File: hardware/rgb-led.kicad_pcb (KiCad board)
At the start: 2 copper layers, 20 x 25 mm, 22 parts, among them P1 CON-SENSOR, Q1 2N7002P, U1 M24C64, U2 DRILL, U3 DRILL, U4 DRILL, U5 DRILL

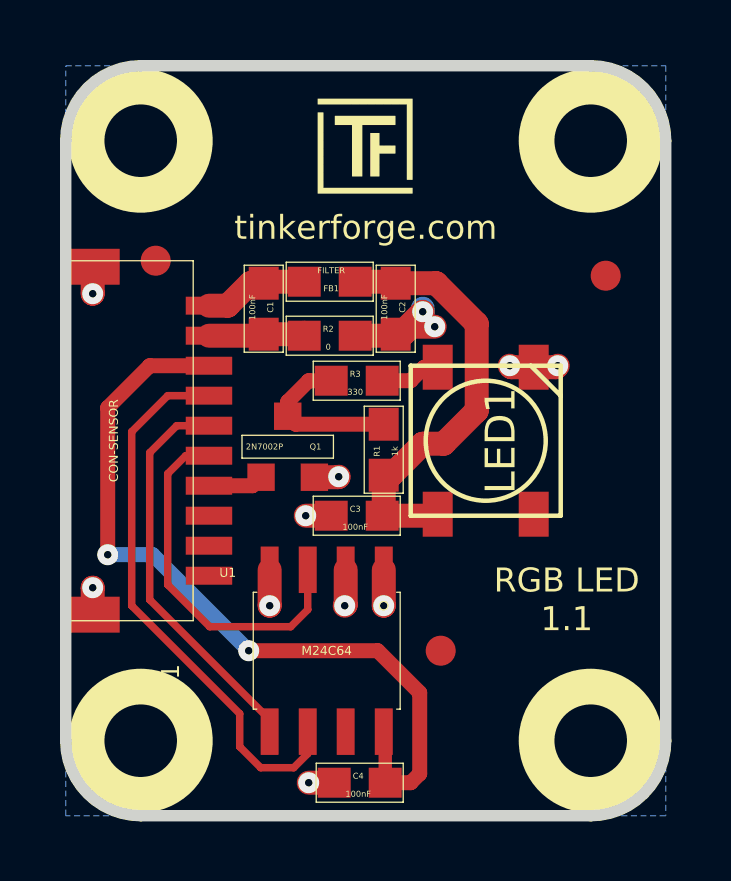
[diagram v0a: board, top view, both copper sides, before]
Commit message: Add 3d information (final)
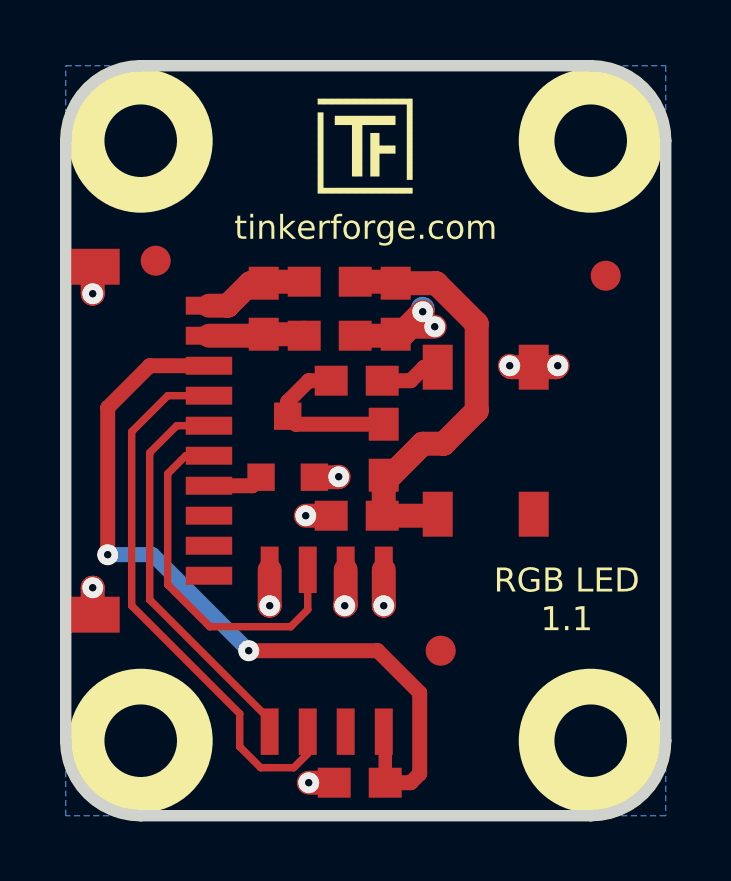
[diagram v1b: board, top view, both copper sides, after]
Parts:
- C1, C2, C3, C4, FB1: footprint kicad-libraries:0603E -> kicad-libraries:C0603E
- R1, R2, R3: footprint kicad-libraries:0603E -> kicad-libraries:R0603E
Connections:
- LED1 pad 2: (no net) -> Net-(LED1-Pad2)
- P1 pad 10: (no net) -> Net-(P1-Pad10)
- P1 pad 8: (no net) -> Net-(P1-Pad8)
- P1 pad 9: (no net) -> Net-(P1-Pad9)
- U1 pad 7: (no net) -> Net-(U1-Pad7)
